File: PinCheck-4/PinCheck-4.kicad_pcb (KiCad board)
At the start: 2 copper layers, 39.2 x 60 mm, 59 parts, among them J1 BatteryHolder, J2 DA15_Socket, J3 LEMHAL Header, Q1 PMOS, SW1 SW_SPST, SW2 SW_SPST, U1 TPS61221DCK, U10 4072, U2 ICM7555xB, U3 4017, U4 TMUX1574DYY, U5 74HC14, U6 74HC14, U7 USBLC6-4SC6, U8 7408, U9 7408

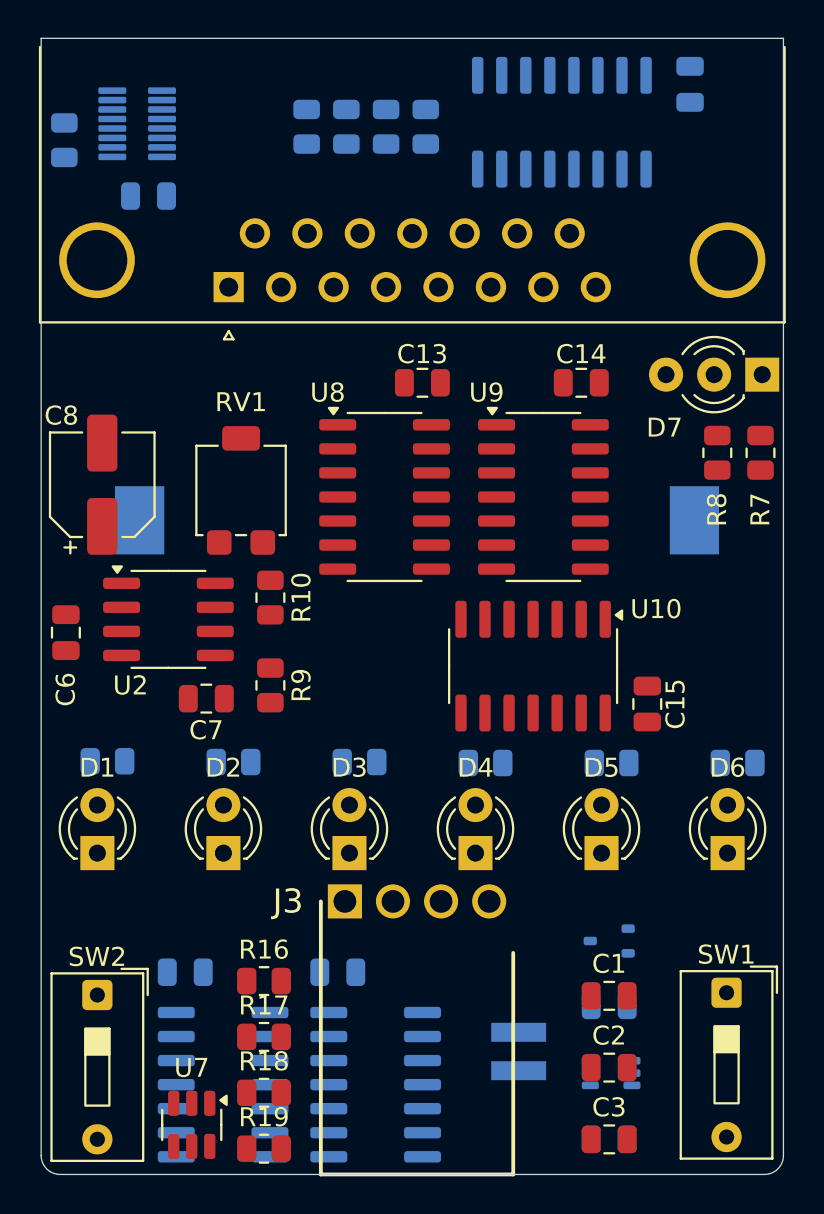
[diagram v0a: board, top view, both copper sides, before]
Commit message: Daily sync 2025-08-30 13:49
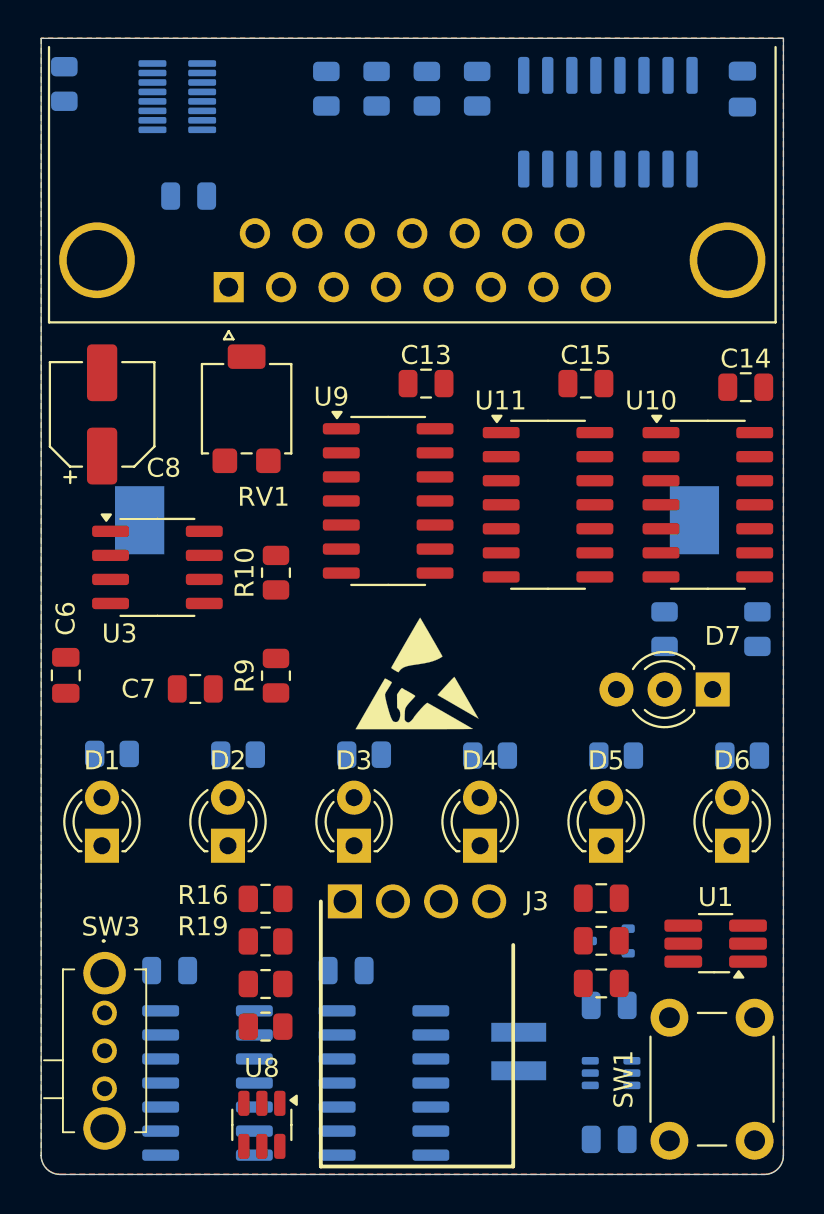
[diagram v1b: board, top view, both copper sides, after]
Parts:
- removed SW2: SW_SPST, Button_Switch_THT:SW_DIP_SPSTx01_Slide_9.78x4.72mm_W7.62mm_P2.54mm
- added REF**: ESD-Logo_6.6x6mm_SilkScreen, Symbol:ESD-Logo_6.6x6mm_SilkScreen, F.Cu at (151.8, 105.1)
- added SW3: OS102011MA1QS1, Button_Switch_THT:OS102011MA1QS1, F.Cu at (135.3, 123.1)
- added U1: MAX16054AZT_T, Package_TO_SOT_SMD:TSOT-23-6_HandSoldering, F.Cu at (167.6, 119.4)
- R7, R8: moved to B.Cu
- SW1: footprint Button_Switch_THT:SW_DIP_SPSTx01_Slide_9.78x4.72mm_W7.62mm_P2.54mm -> Button_Switch_THT:SW_PUSH_6mm
- moved C15 17.2 mm to (160.7, 89.9), turned to 180 degrees
- moved D7 16.8 mm to (167.4, 106.0)
- moved R8 9.72 mm to (164.9, 102.8), turned to 90 degrees
- moved R7 9.31 mm to (169.8, 102.8), turned to 90 degrees
- moved U10 8.69 mm to (167.2, 96.3)
- moved C14 8.69 mm to (169.2, 90.0)
- moved U11 8.56 mm to (158.7, 96.3), turned to 0 degrees
- moved C3 8.25 mm to (161.5, 121.5)
- moved C2 6.71 mm to (161.5, 119.3)
- moved R19 6.44 mm to (143.8, 123.8)
- moved R18 5.74 mm to (143.8, 121.6)
- moved C1 5.17 mm to (161.5, 117.0)
- moved R17 5.04 mm to (143.8, 119.3)
- moved R16 4.34 mm to (143.8, 117.1)
- moved RV1 4.32 mm to (142.8, 91.2)
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- renumbered U9 to U10, U10 to U11, U1 to U2, U2 to U3, U3 to U4, U4 to U5, U5 to U6, U6 to U7, U7 to U8, U8 to U9
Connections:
- J1 pad 1: Net-(J1-Pin_1) -> +BATT
- SW1 pad 1: Net-(J1-Pin_1) -> GND
- SW1 pad 2: Net-(Q1-S) -> Net-(SW1-B)
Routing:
- added copper zone on B.Cu, net GND
- added copper zone on F.Cu, net GND
